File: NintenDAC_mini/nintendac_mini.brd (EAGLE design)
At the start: 26 x 42 mm, 31 parts, among them IC1 STM32F10XCXT6, IC3 24C64ST, X1 USB-MICROB

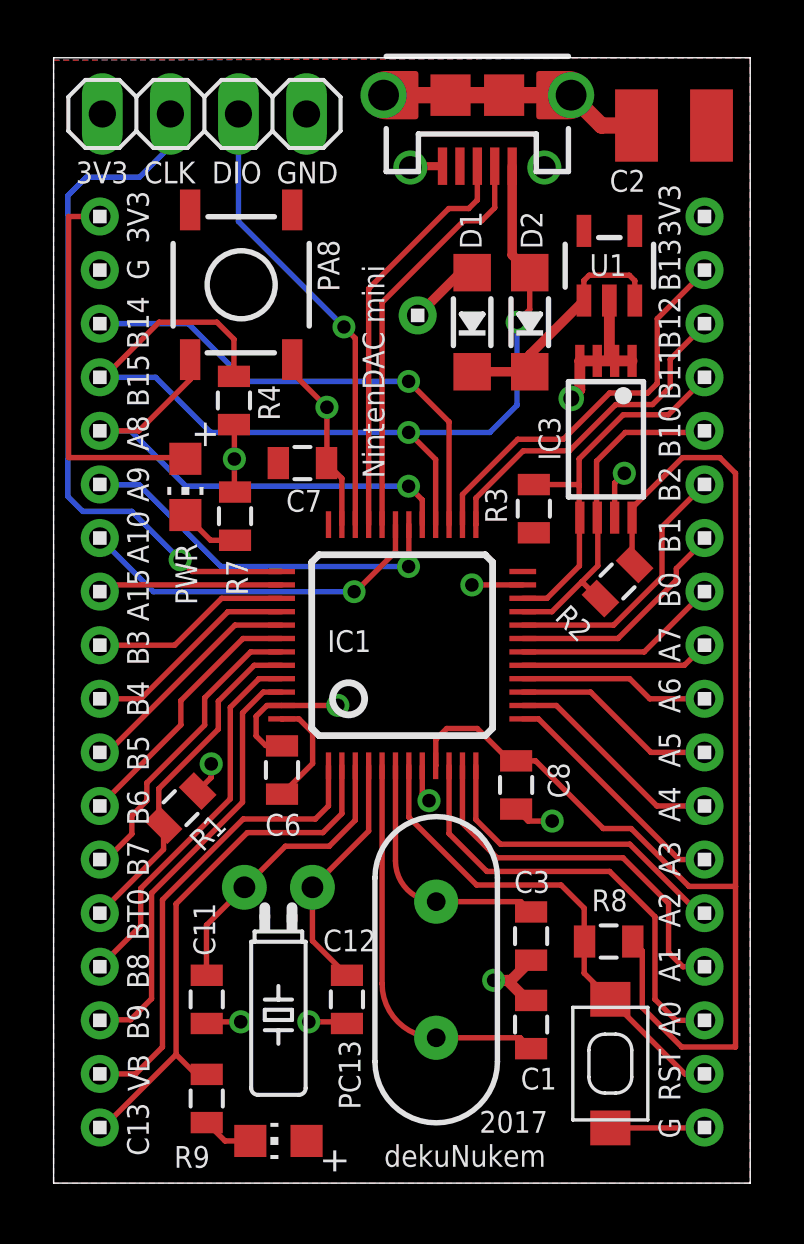
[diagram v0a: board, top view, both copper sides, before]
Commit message: board cleanup
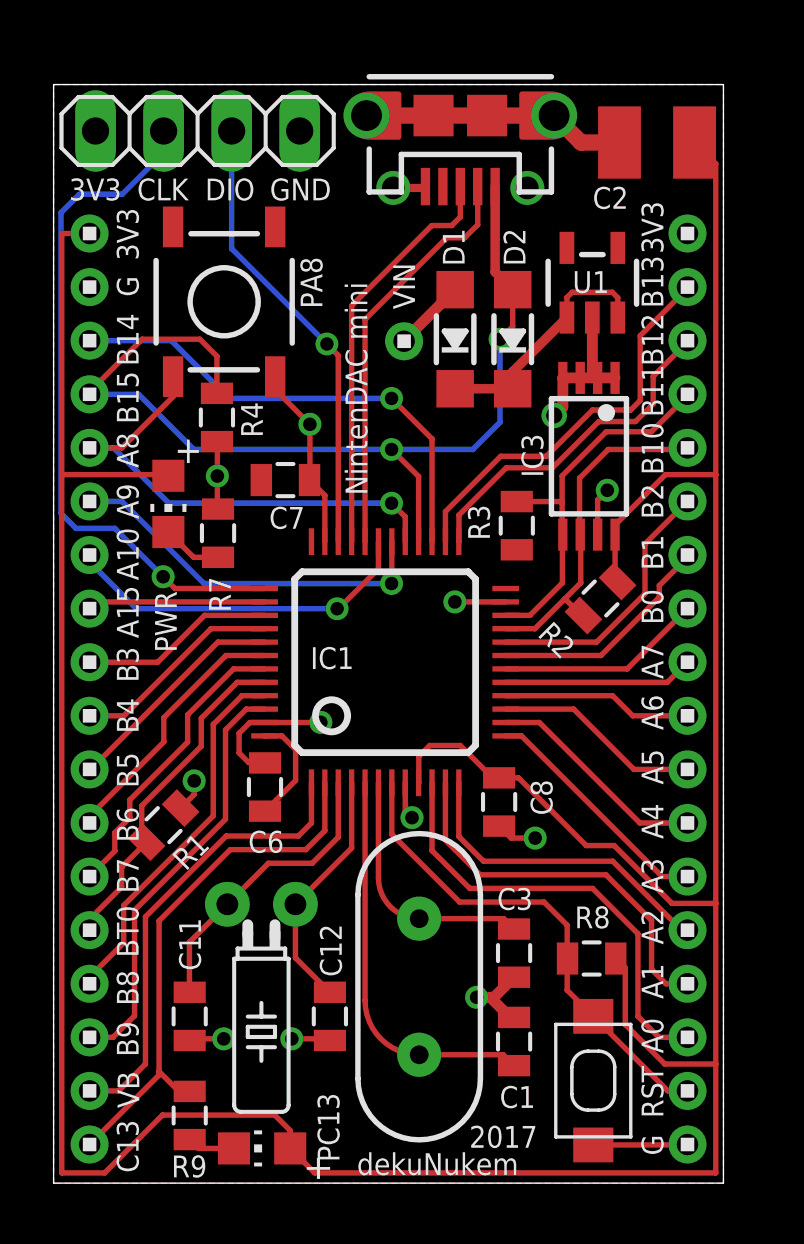
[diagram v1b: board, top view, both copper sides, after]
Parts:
- moved U$3 1.09 mm to (13.1, 31.4)
- moved X1 0.99 mm to (15.2, 39.8)
- moved C2 0.90 mm to (22.5, 38.8)
- moved C7 0.90 mm to (8.65, 26.2)
- moved D2 0.90 mm to (17.1, 31.5)
- moved IC3 0.90 mm to (20.0, 27.1)
- moved R2 0.90 mm to (20.4, 21.8)
- moved Y1 0.90 mm to (13.6, 7.33)
- moved C1 0.90 mm to (17.2, 5.28)
- moved C3 0.90 mm to (17.2, 8.59)
- moved D1 0.90 mm to (15.0, 31.5)
- moved IC1 0.90 mm to (12.4, 19.4)
- moved PWR 0.90 mm to (4.28, 25.3)
- moved R4 0.90 mm to (6.10, 28.6)
- moved C6 0.90 mm to (7.89, 14.8)
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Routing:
- net +3V3: track 68.7 -> 137.6 mm
- net N$9: track 26.2 -> 25.6 mm
- net N$45: track 37.6 -> 37.0 mm
- net N$43: track 18.9 -> 18.4 mm
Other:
- board size 26 x 42 mm -> 25 x 41 mm
- board text added: "VIN"
